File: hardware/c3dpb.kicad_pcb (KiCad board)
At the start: 4 copper layers, 76 x 55 mm, 332 parts, among them IC1 TMC2209, IC2 TMC2209, IC3 TMC2209, IC4 TMC2209, J1 Conn_01x01, J10 Conn_01x04, J100 Conn_01x01, J101 Conn_01x01, J102 Conn_01x01, J2 Conn_01x01, J24 Conn_01x01, J3 Conn_01x01, J39 Screw_Terminal_01x02, J4 Conn_01x01, J44 Conn_01x01, J45 Conn_01x01, J46 Conn_01x03, J47 Conn_01x03, J48 Conn_01x01, J49 Conn_01x01, J5 Conn_01x01, J50 Conn_01x01, J51 Conn_01x01, J53 Conn_01x01, J54 Conn_01x01, J55 Conn_01x01, J56 Conn_01x01, J57 Conn_01x01, J58 Conn_01x01, J59 Conn_01x01, J6 Conn_01x01, J60 USB_C_Receptacle, J62 Conn_01x02, J66 Conn_01x03, J67 Conn_01x03, J68 Conn_01x01, J69 Conn_01x01, J7 Conn_01x04, J70 Conn_01x01, J71 Conn_01x02, J72 Conn_01x02, J73 Conn_01x02, J74 Conn_01x02, J79 Conn_01x03, J8 Conn_01x04, J80 Conn_01x03, J81 Conn_01x03, J82 Screw_Terminal_01x04, J83 Conn_01x03, J84 Conn_01x03, J85 Conn_01x03, J86 Conn_01x03, J87 Conn_01x03, J9 Conn_01x04, J94 Conn_01x01, J95 Conn_01x01, J96 Conn_01x01, J98 Conn_01x01, J99 Conn_01x01, Q1 AON7418, Q10 AO3400, Q12 AO3400, Q13 AO3400, Q2 AO3400, Q3 AO3400, Q4 AO3400, Q5 AO3400, Q6 AON7418, Q7 AON7418, Q8 AO3400, Q9 AO3400, SW1 3x6mm, SW2 3x6mm, U1 ATSAMD51J19A-M, U2 LM1117-3.3, U3 SY8303, U4 SY8303, U5 MAX6675, U7 IR4427S

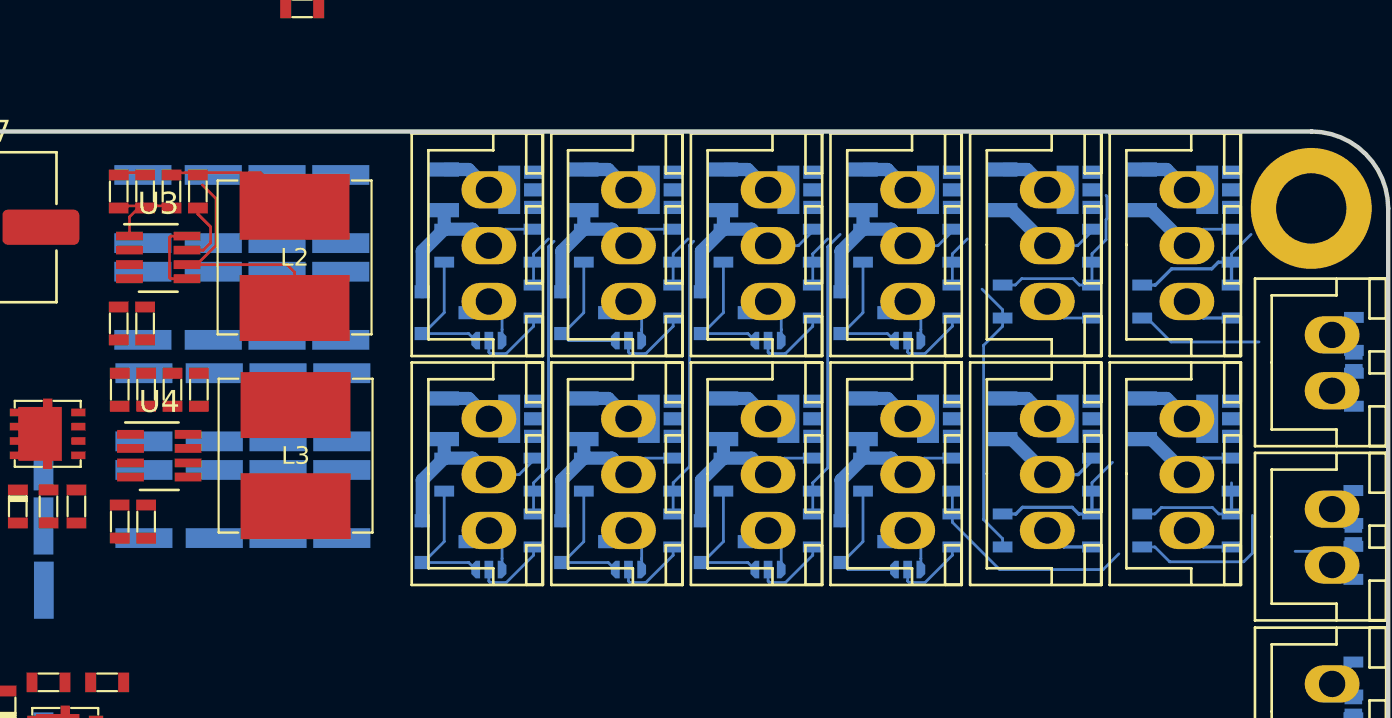
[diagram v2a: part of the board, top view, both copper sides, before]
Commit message: layout
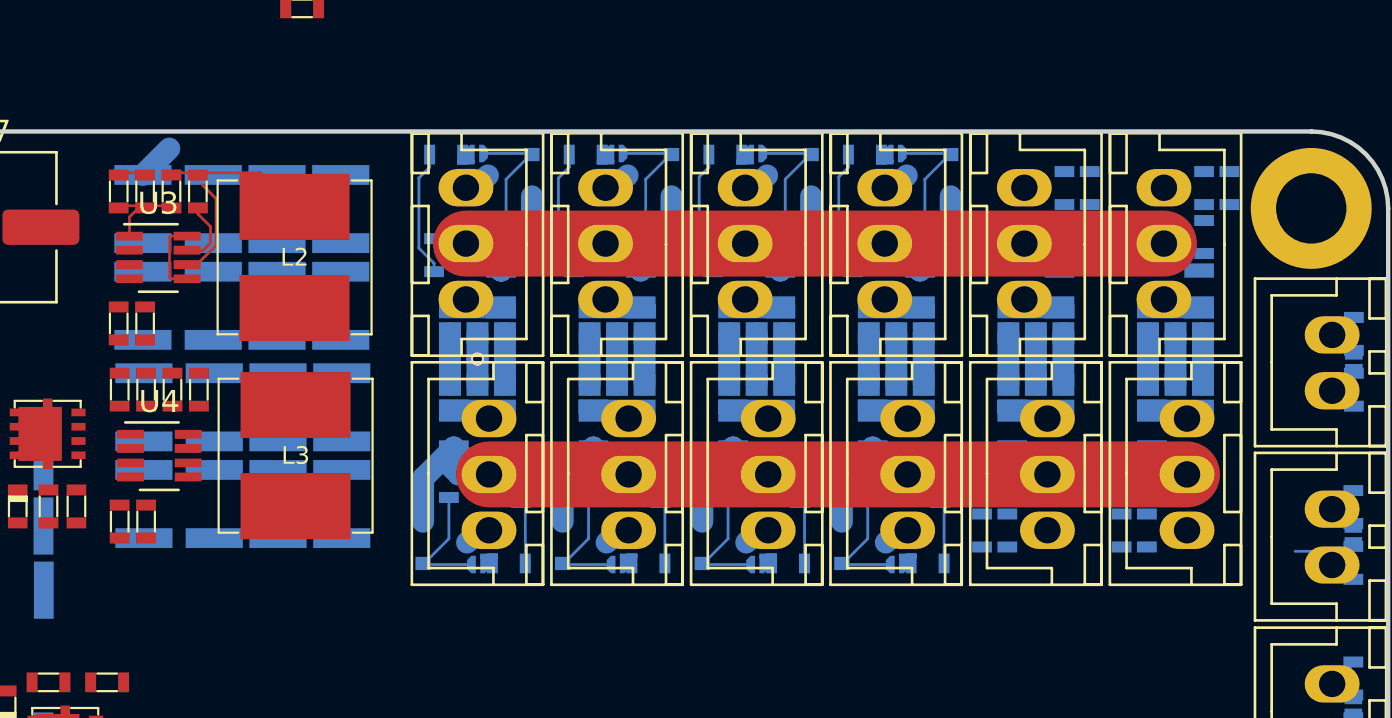
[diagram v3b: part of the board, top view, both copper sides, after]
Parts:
- removed JP28, JP29, JP30, JP34, JP35: SolderJumper_3_Open, _Generic:Solder Jumper 3P
- added JP10: SolderJumper_2_Open, _Generic:Solder Jumper 2P, B.Cu at (153.6, 51.0)
- added JP11: SolderJumper_2_Open, _Generic:Solder Jumper 2P, B.Cu at (146.8, 51.6)
- added JP12: SolderJumper_2_Open, _Generic:Solder Jumper 2P, B.Cu at (147.8, 69.1)
- added JP13: SolderJumper_2_Open, _Generic:Solder Jumper 2P, B.Cu at (153.1, 51.6)
- added JP14: SolderJumper_2_Open, _Generic:Solder Jumper 2P, B.Cu at (134.6, 51.0)
- added JP2: SolderJumper_2_Open, _Generic:Solder Jumper 2P, B.Cu at (153.7, 69.7)
- added JP3: SolderJumper_2_Open, _Generic:Solder Jumper 2P, B.Cu at (140.9, 51.0)
- added JP4: SolderJumper_2_Open, _Generic:Solder Jumper 2P, B.Cu at (140.9, 69.7)
- added JP5: SolderJumper_2_Open, _Generic:Solder Jumper 2P, B.Cu at (154.2, 69.1)
- added JP6: SolderJumper_2_Open, _Generic:Solder Jumper 2P, B.Cu at (140.4, 51.6)
- added JP7: SolderJumper_2_Open, _Generic:Solder Jumper 2P, B.Cu at (141.4, 69.1)
- added JP8: SolderJumper_2_Open, _Generic:Solder Jumper 2P, B.Cu at (147.2, 51.0)
- added JP9: SolderJumper_2_Open, _Generic:Solder Jumper 2P, B.Cu at (147.3, 69.7)
- JP22, JP23, JP24: value SolderJumper_3_Open -> SolderJumper_2_Open; footprint _Generic:Solder Jumper 3P -> _Generic:Solder Jumper 2P
- moved JP22 19.5 mm to (134.6, 69.7)
- moved JP23 10.8 mm to (134.1, 51.6), turned to 270 degrees
- moved R69 7.78 mm to (152.2, 51.0), turned to 0 degrees
- moved R57 7.78 mm to (139.5, 51.0), turned to 0 degrees
- moved R65 7.78 mm to (145.8, 51.0), turned to 0 degrees
- moved R71 7.78 mm to (133.2, 51.0), turned to 0 degrees
- moved Q10 6.92 mm to (155.1, 52.0), turned to 180 degrees
- moved Q12 6.92 mm to (136.1, 52.0), turned to 180 degrees
- moved Q4 6.92 mm to (142.4, 52.0), turned to 180 degrees
- moved Q8 6.92 mm to (148.8, 52.0), turned to 180 degrees
- moved R36 6.51 mm to (162.4, 52.6), turned to 270 degrees
- moved R40 6.51 mm to (168.8, 52.6), turned to 270 degrees
- moved JP24 6.40 mm to (135.1, 69.1), turned to 90 degrees
- moved JP17 6.29 mm to (160.0, 58.6), turned to 90 degrees
- moved JP26 6.29 mm to (140.9, 58.6), turned to 90 degrees
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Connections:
- JP22 pad 1: Net-(J79-Pad3) -> Net-(JP22-Pad1)
- JP23 pad 1: Net-(J80-Pad3) -> Net-(JP14-Pad1)
- JP23 pad 2: Net-(JP23-Pad2) -> Net-(J86-Pad3)
- JP24 pad 1: Net-(J81-Pad3) -> Net-(JP22-Pad1)
- JP24 pad 2: Net-(JP24-Pad2) -> Net-(J87-Pad3)
- JP25 pad 2: +5V -> +24V
- JP25 pad 4: +24V -> +5V
- JP27 pad 2: +5V -> +24V
- JP27 pad 4: +24V -> +5V
- JP32 pad 2: +5V -> +24V
- JP32 pad 4: +24V -> +5V
- JP37 pad 2: +5V -> +24V
- JP37 pad 4: +24V -> +5V
- JP43 pad 2: +5V -> +24V
- JP43 pad 4: +24V -> +5V
- JP44 pad 2: +5V -> +24V
- JP44 pad 4: +24V -> +5V
- Q13 pad 1: Net-(JP35-Pad3) -> Net-(JP22-Pad2)
- Q3 pad 1: Net-(JP22-Pad3) -> Net-(JP2-Pad2)
- Q4 pad 1: Net-(JP23-Pad3) -> Net-(JP3-Pad2)
- Q5 pad 1: Net-(JP24-Pad3) -> Net-(JP4-Pad2)
- R55 pad 2: Net-(JP22-Pad2) -> Net-(JP2-Pad1)
- R56 pad 2: Net-(JP22-Pad3) -> Net-(JP2-Pad2)
- R57 pad 2: Net-(JP23-Pad2) -> Net-(JP3-Pad1)
- R58 pad 2: Net-(JP23-Pad3) -> Net-(JP3-Pad2)
- R59 pad 2: Net-(JP24-Pad2) -> Net-(JP4-Pad1)
- R60 pad 2: Net-(JP24-Pad3) -> Net-(JP4-Pad2)
- R71 pad 2: Net-(JP34-Pad2) -> Net-(JP14-Pad1)
- R73 pad 2: Net-(JP35-Pad2) -> Net-(JP22-Pad1)
- R74 pad 2: Net-(JP35-Pad3) -> Net-(JP22-Pad2)
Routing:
- net GND: track 246.5 -> 296.8 mm
- net +3V3: track 26.3 -> 0.50 mm
- net +24V: track 113.3 -> 129.1 mm
- net +12V: track 6.24 -> 21.3 mm, vias 0 -> 1
- net +5V: track 0.00 -> 14.1 mm
- net /P1.28_ADV: track 13.2 -> 2.86 mm
- net /P1.25_ADV: track 12.8 -> 2.86 mm
- net /P1.19_ADV: track 12.8 -> 2.86 mm
- net /P0.0_END: track 8.68 -> 0.00 mm
- net /P0.20_END: track 7.77 -> 0.00 mm
- net /P0.22_ADV: track 10.2 -> 2.86 mm
- net /P0.1_END: track 7.05 -> 0.00 mm
- net Net-(C37-Pad2): track 11.4 -> 4.69 mm
- net Net-(JP22-Pad3): track 6.26 -> 0.00 mm
- net Net-(JP24-Pad3): track 6.26 -> 0.00 mm
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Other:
- board text removed: "P0.0"
- board text removed: "P0.1"
- board text removed: "P0.19"
- board text removed: "P0.20"
- board text removed: "P0.22"
- board text removed: "P0.28"
- board text removed: "P1.18"
- board text removed: "P1.19"
- board text removed: "P1.22"
- board text removed: "P1.25"
- board text removed: "P1.26"
- board text removed: "P1.29"

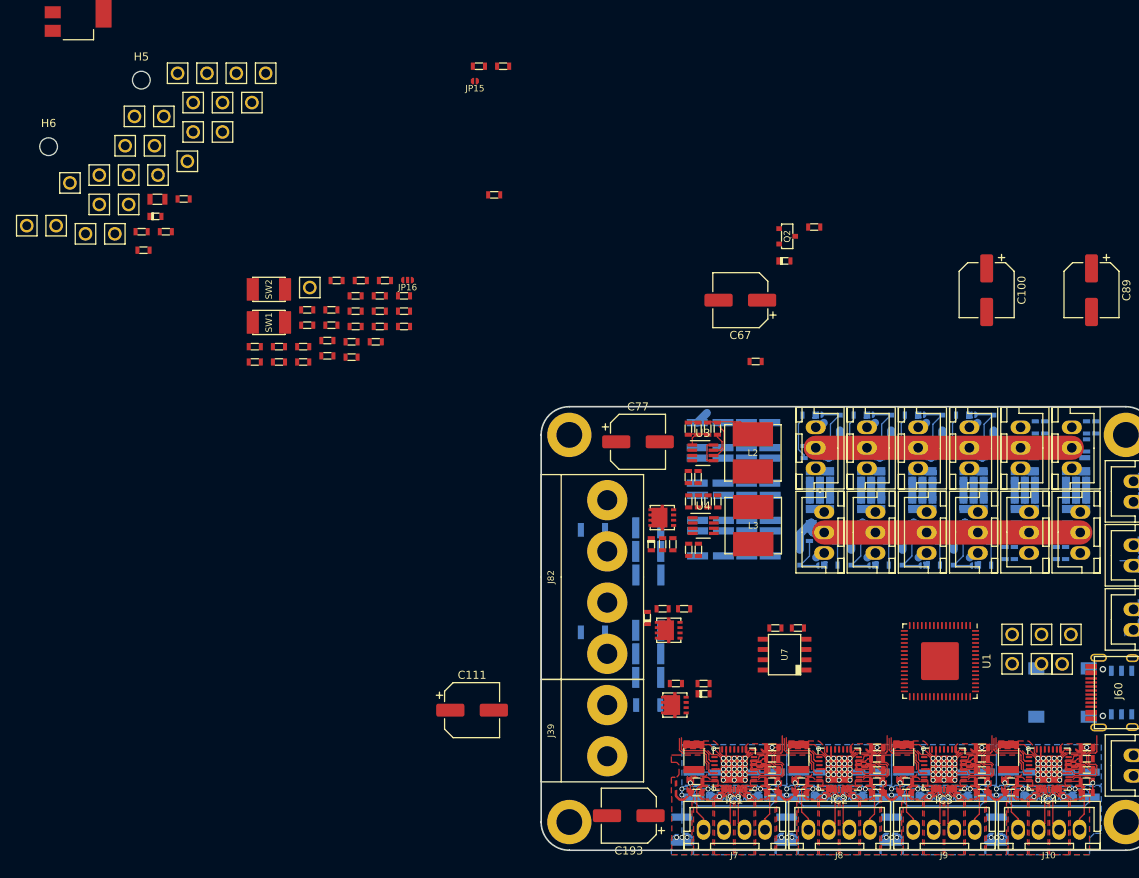
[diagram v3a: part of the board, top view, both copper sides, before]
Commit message: combine
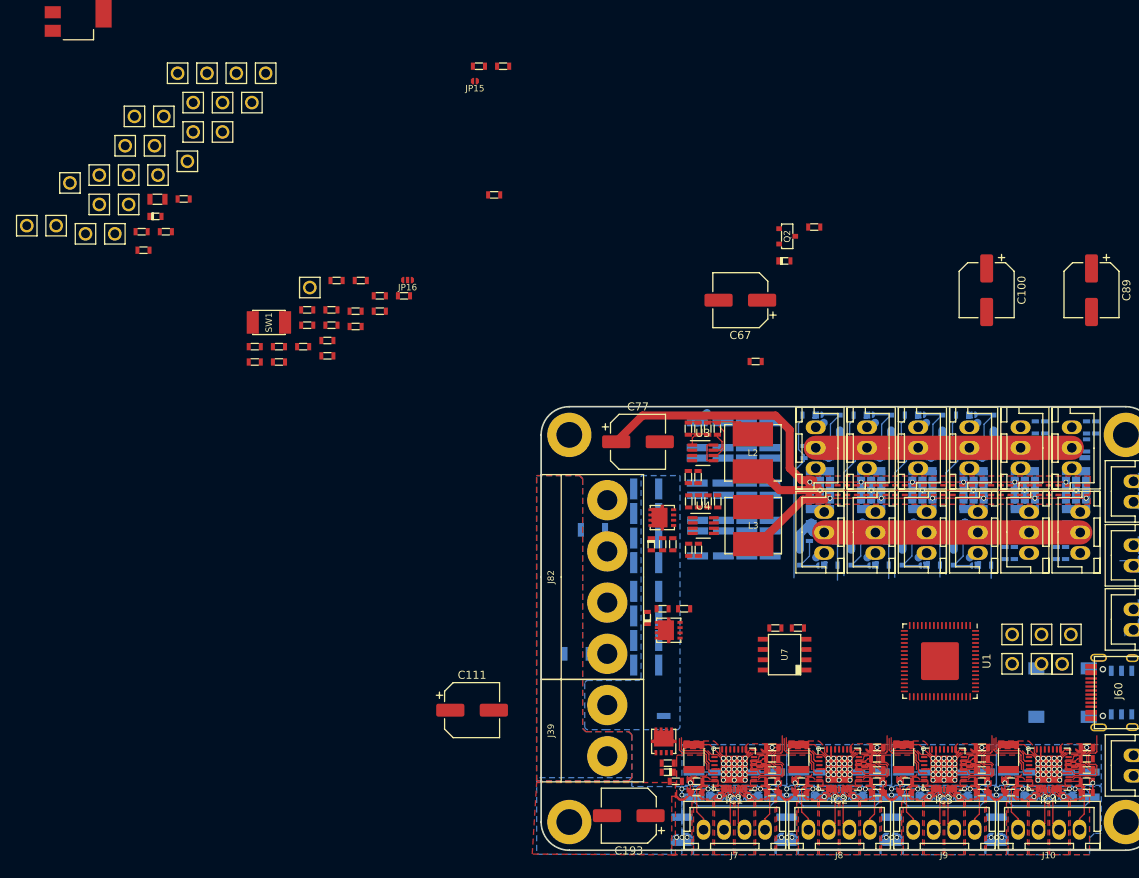
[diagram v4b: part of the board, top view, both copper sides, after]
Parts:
- removed C17: 10u, _Generic:0603_CAP
- removed H5, H6: MountingHole, MountingHole:MountingHole_2.2mm_M2_DIN965
- removed R2: 10k, _Generic:0603_RES
- removed R3, R4, R5: 1k, _Generic:0603_RES
- removed R6, R7: 2.2R, _Generic:0603_RES
- removed SW2: 3x6mm, _Generic:Switch_3x4mm
- C15, C16: value 100n -> 4.7u; footprint _Generic:0603_CAP -> _Generic:1210_CAP; moved to B.Cu
- moved C16 51.2 mm to (113.0, 72.9)
- moved C15 43.3 mm to (113.0, 60.2)
- moved R8 12.1 mm to (116.7, 96.5), turned to 180 degrees
- moved R9 10.8 mm to (115.7, 94.2), turned to 180 degrees
- moved D1 10.7 mm to (115.7, 95.3), turned to 180 degrees
- moved C69 7.62 mm to (113.0, 63.2)
- moved C68 7.62 mm to (113.0, 75.9)
- moved Q1 4.71 mm to (115.2, 91.5), turned to 90 degrees
- moved F1 3.44 mm to (115.2, 89.8), turned to 90 degrees
- moved F3 3.35 mm to (104.4, 80.6)
- moved C74 1.42 mm to (113.0, 82.0)
- moved C79 1.42 mm to (113.0, 69.3)
- moved C192 1.30 mm to (113.0, 79.0)
- moved C73 1.30 mm to (113.0, 66.3)
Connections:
- C15 pad 1: /VREFN -> Net-(C15-Pad1)
- C15 pad 2: /VREFP -> DCIN-
- C16 pad 1: /VDDA -> Net-(C16-Pad1)
- C16 pad 2: /VSSA -> DCIN-
- C192 pad 1: Net-(C192-Pad1) -> Net-(C16-Pad1)
- C68 pad 1: Net-(C192-Pad1) -> Net-(C16-Pad1)
- C69 pad 1: Net-(C69-Pad1) -> Net-(C15-Pad1)
- C73 pad 1: Net-(C69-Pad1) -> Net-(C15-Pad1)
- C74 pad 1: Net-(C192-Pad1) -> Net-(C16-Pad1)
- C79 pad 1: Net-(C69-Pad1) -> Net-(C15-Pad1)
- F2 pad 1: Net-(C69-Pad1) -> Net-(C15-Pad1)
- F3 pad 1: Net-(C192-Pad1) -> Net-(C16-Pad1)
- J82 pad 2: Net-(C69-Pad1) -> Net-(C15-Pad1)
- J82 pad 4: Net-(C192-Pad1) -> Net-(C16-Pad1)
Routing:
- net +24V: track 129.1 -> 192.7 mm, vias 24 -> 30
- net +5V: track 14.1 -> 57.0 mm, vias 0 -> 6
- net +12V: track 21.3 -> 62.3 mm, vias 1 -> 6
- net /P1.26_ADV: track 5.77 -> 21.2 mm
- net /P1.18_ADV: track 5.81 -> 21.2 mm
- net /P1.22_ADV: track 5.81 -> 21.0 mm
- net /P1.29_ADV: track 5.77 -> 20.8 mm
- net /P1.19_ADV: track 2.86 -> 4.73 mm
- net /P1.25_ADV: track 2.86 -> 4.51 mm
- net /P0.22_ADV: track 2.86 -> 4.51 mm
- net /P1.28_ADV: track 2.86 -> 4.33 mm
- added copper zone on F.Cu, net +12V
- added copper zone on F.Cu, net +5V
- added copper zone on B.Cu, net DCIN-
